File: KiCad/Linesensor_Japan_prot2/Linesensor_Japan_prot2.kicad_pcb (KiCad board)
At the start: 2 copper layers, 197.2 x 140 mm, 147 parts, among them J1 Conn_01x04_Socket, J2 Conn_01x02_Socket, J3 Conn_01x09_Socket, J4 Conn_01x09_Socket, Q1 Q_Photo_NPN, Q10 Q_Photo_NPN, Q11 Q_Photo_NPN, Q12 Q_Photo_NPN, Q13 Q_Photo_NPN, Q14 Q_Photo_NPN, Q15 Q_Photo_NPN, Q16 Q_Photo_NPN, Q17 Q_Photo_NPN, Q18 Q_Photo_NPN, Q19 Q_Photo_NPN, Q2 Q_Photo_NPN, Q20 Q_Photo_NPN, Q21 Q_Photo_NPN, Q22 Q_Photo_NPN, Q23 Q_Photo_NPN, Q24 Q_Photo_NPN, Q25 Q_Photo_NPN, Q26 Q_Photo_NPN, Q27 Q_Photo_NPN, Q28 Q_Photo_NPN, Q29 Q_Photo_NPN, Q3 Q_Photo_NPN, Q30 Q_Photo_NPN, Q31 Q_Photo_NPN, Q32 Q_Photo_NPN, Q33 Q_NMOS, Q4 Q_Photo_NPN, Q5 Q_Photo_NPN, Q6 Q_Photo_NPN, Q7 Q_Photo_NPN, Q8 Q_Photo_NPN, Q9 Q_Photo_NPN, U1 CD74HC4067SM, U2 CD74HC4067SM

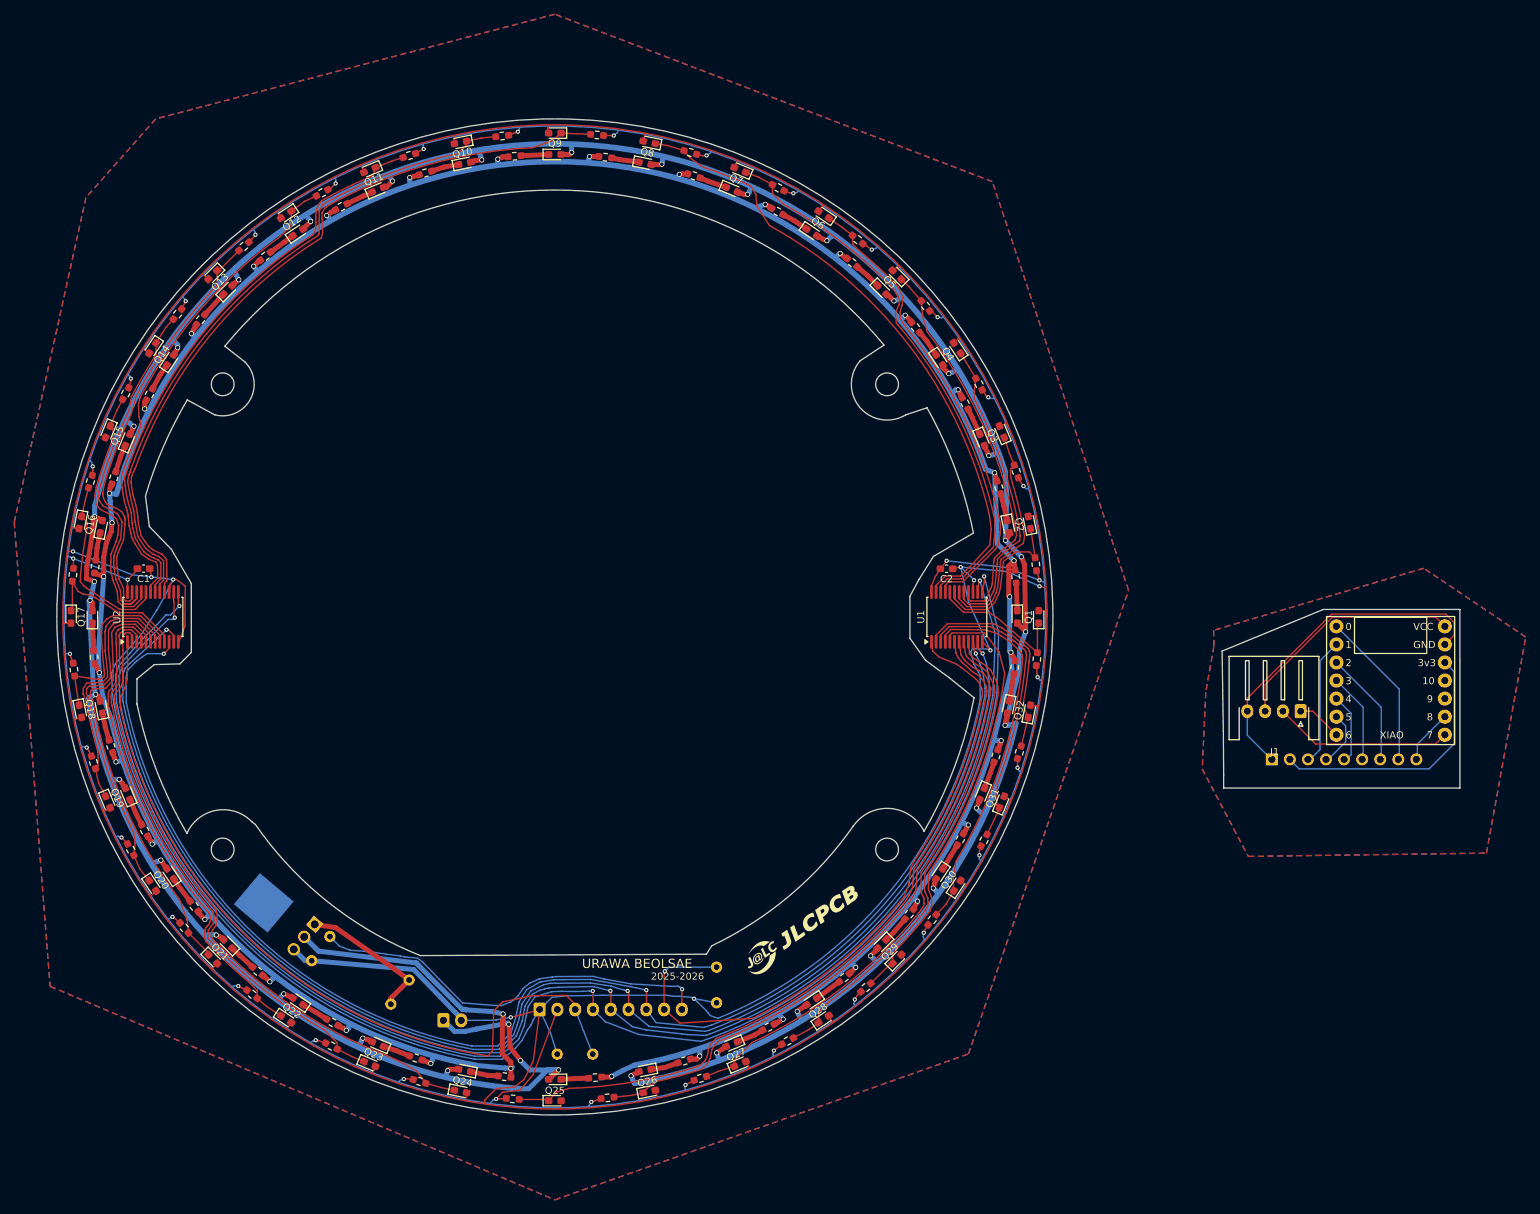
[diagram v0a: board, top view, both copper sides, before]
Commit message: ああああああああああああああああああ
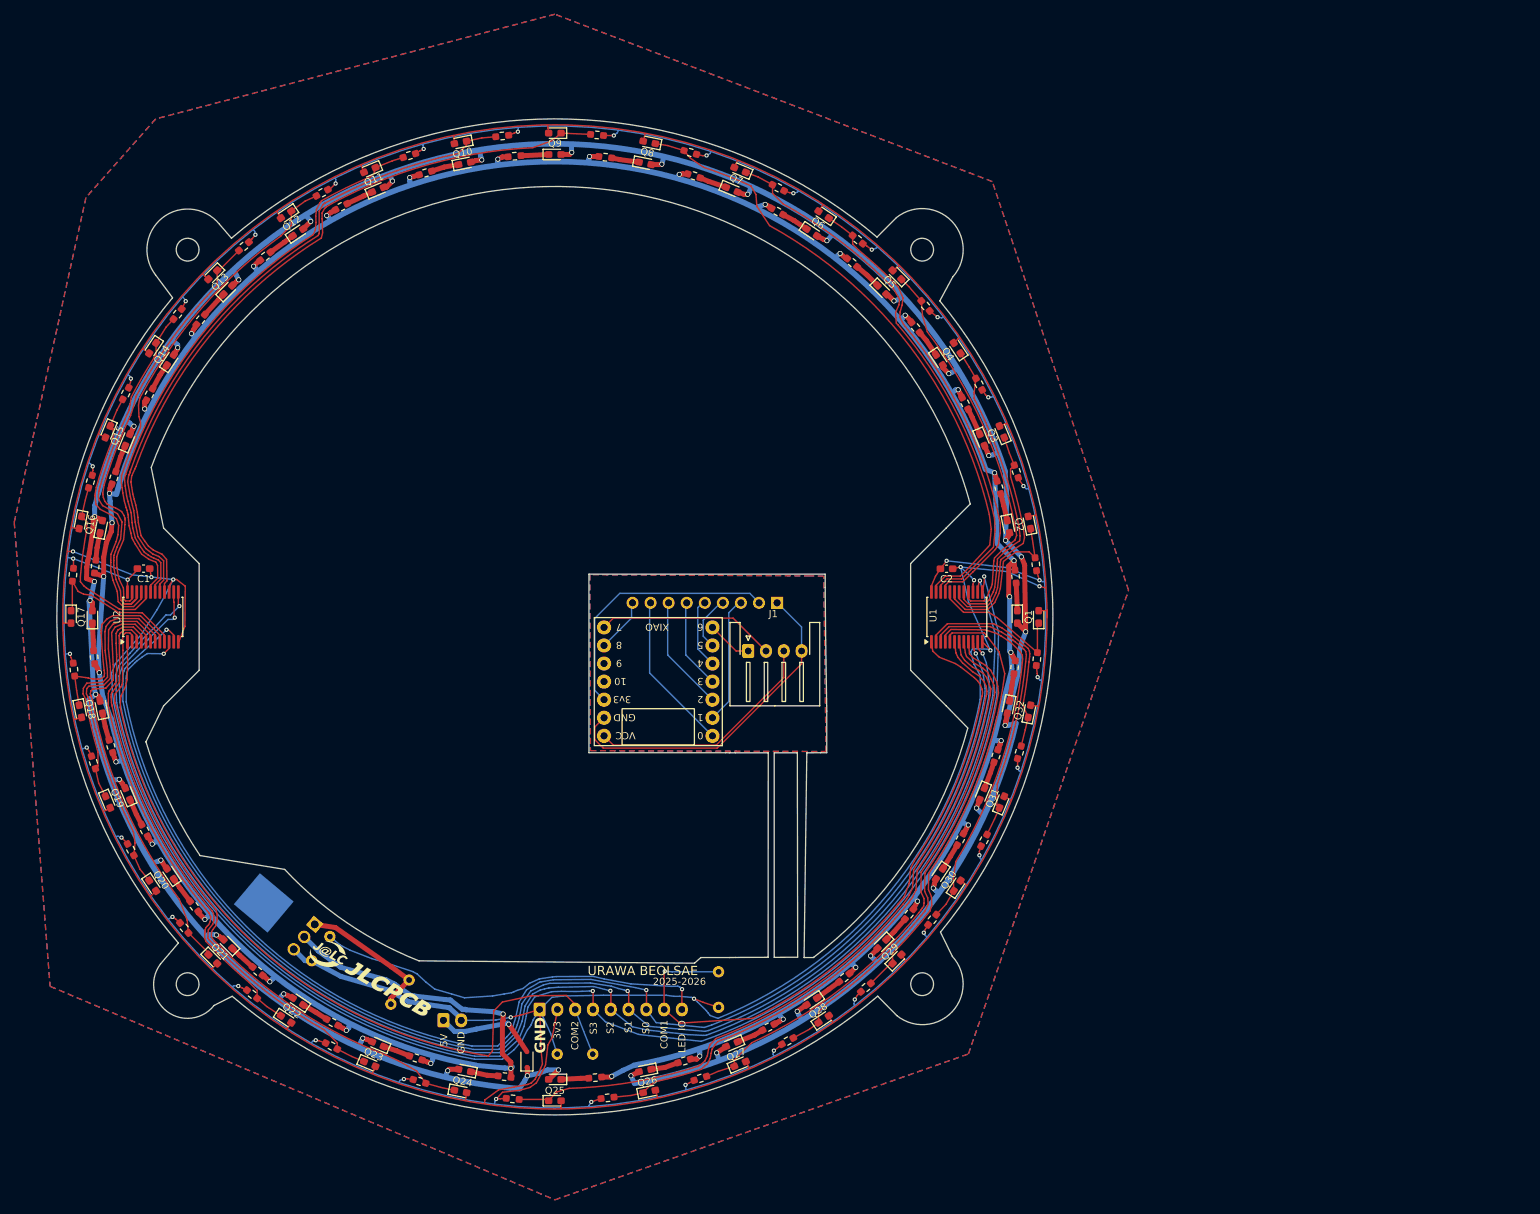
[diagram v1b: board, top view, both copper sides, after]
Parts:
- added REF**: D_SOD-323F, Diode_SMD:D_SOD-323F, F.Cu at (96.1, 162.2)
- moved H6 129.5 mm to (151.6, 151.6)
- moved U3 102.9 mm to (114.5, 109.1), turned to 180 degrees
- moved H1 100.1 mm to (48.4, 151.6)
- moved H4 84.5 mm to (48.4, 48.4)
- moved J1 78.1 mm to (127.2, 104.8), turned to 0 degrees
- moved J3 72.9 mm to (131.2, 98.0), turned to 90 degrees
- moved G*** 60.9 mm to (74.0, 150.8), turned to -30 degrees
- moved H2 19.6 mm to (151.6, 48.4)
- moved C3 0.71 mm to (123.0, 149.9)
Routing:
- net LED_5V: track 167.2 -> 161.4 mm
- net LED_IO: track 65.1 -> 63.1 mm
- net Net-(Q33-D): track 175.7 -> 175.0 mm
- net 3v3: track 151.7 -> 151.1 mm
- net GND: track 279.2 -> 279.8 mm
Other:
- board size 197.2 x 140 mm -> 140 x 140 mm
- board text added: "3v3"
- board text added: "5V"
- board text added: "COM1"
- board text added: "COM2"
- board text added: "GND"
- board text added: "LED IO"
- board text added: "S0"
- board text added: "S1"
- board text added: "S2"
- board text added: "S3"
